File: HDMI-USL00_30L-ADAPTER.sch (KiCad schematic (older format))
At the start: 9 parts, among them J1 1747981-1, J2 USL00-30L, J3 USL00-30L, J4 53261-0471

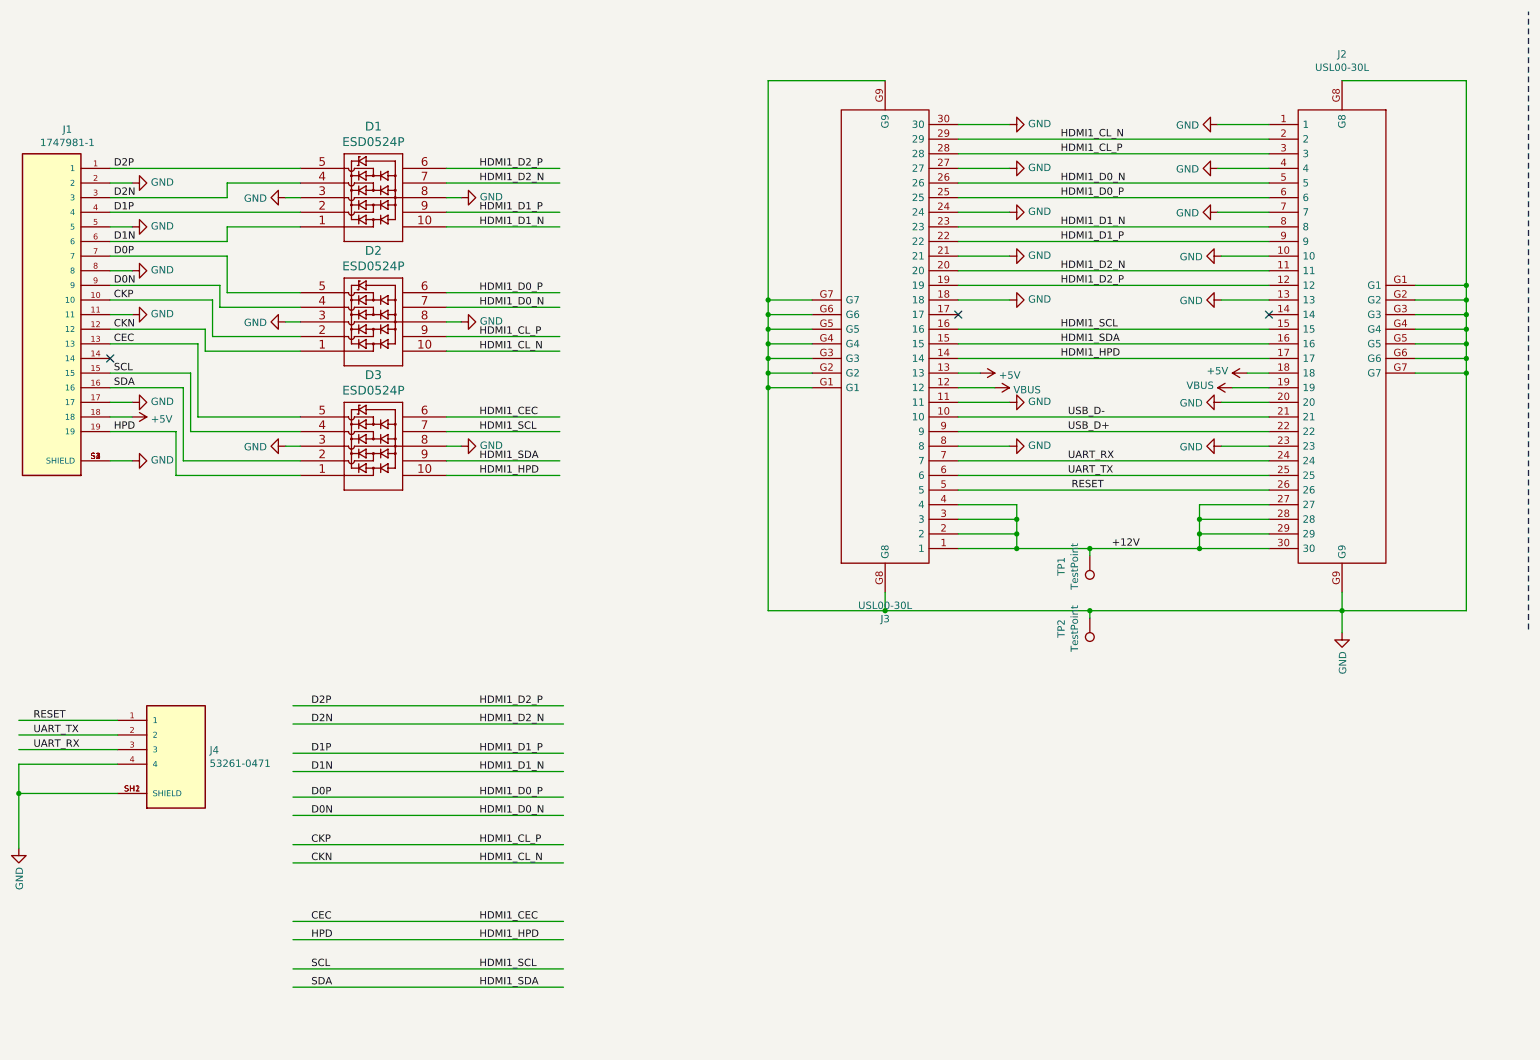
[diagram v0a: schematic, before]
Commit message: Add production data for release V1A
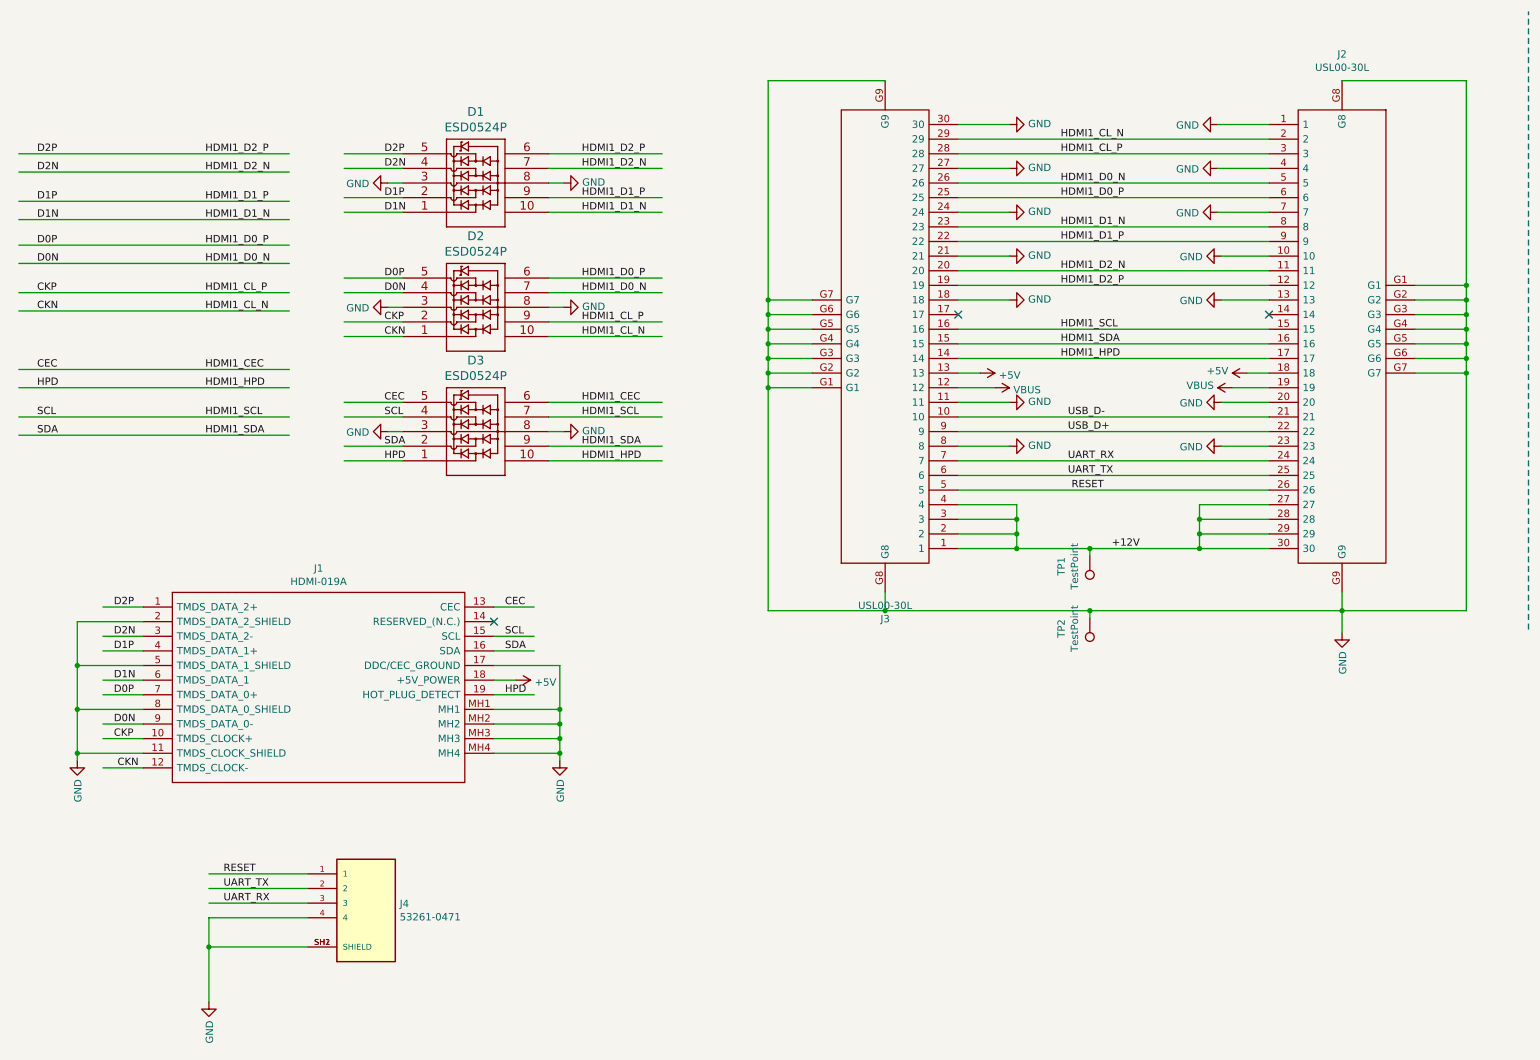
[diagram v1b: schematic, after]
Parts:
- removed J1: 1747981-1, footprints:TE_1747981-1, symbol 1747981-1:1747981-1
- added J1: HDMI-019A, HDMI019A, symbol HDMI-019A:HDMI-019A
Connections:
- wire segments 167 -> 171
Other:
- moved on the sheet: D1, D2, D3, J4
